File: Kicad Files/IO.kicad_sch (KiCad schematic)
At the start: 1 part, among them U46 RP2040

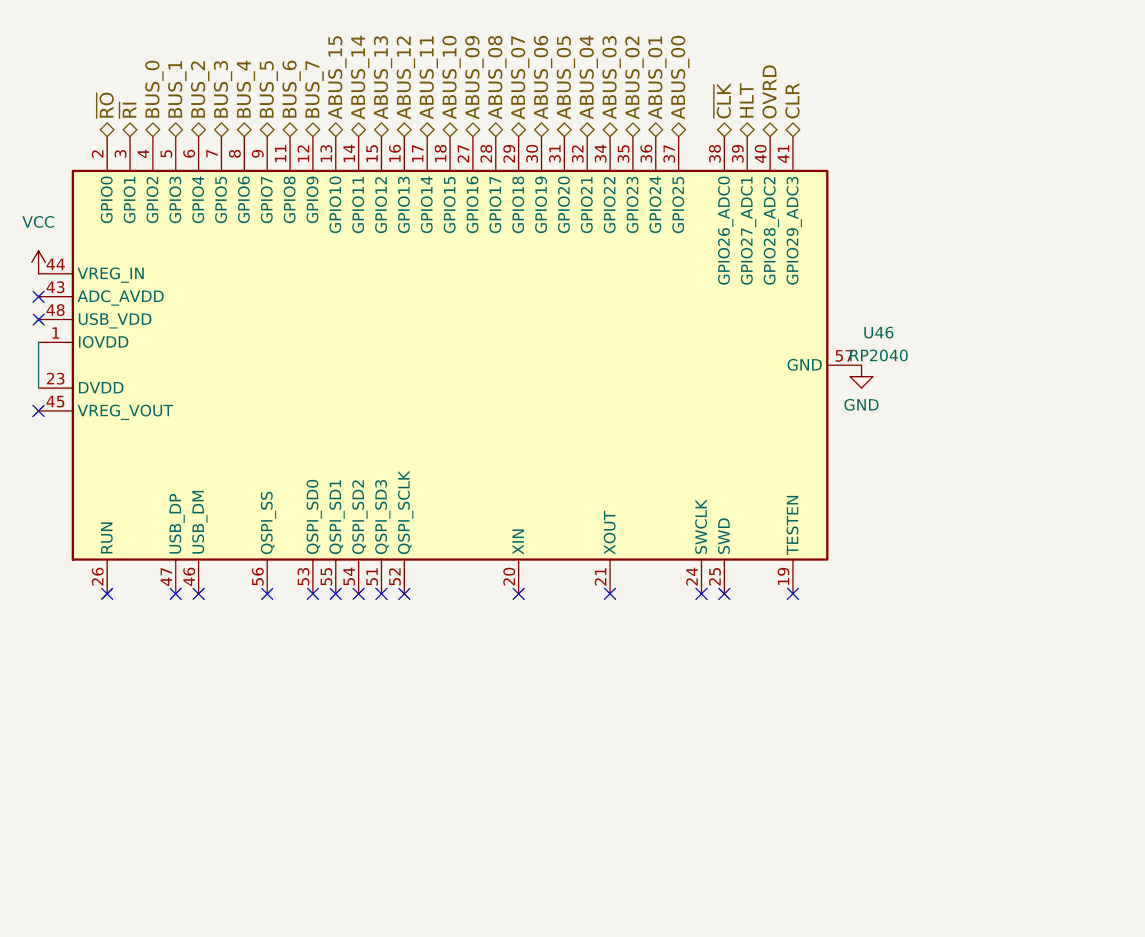
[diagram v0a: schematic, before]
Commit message: im sooo stupiiid
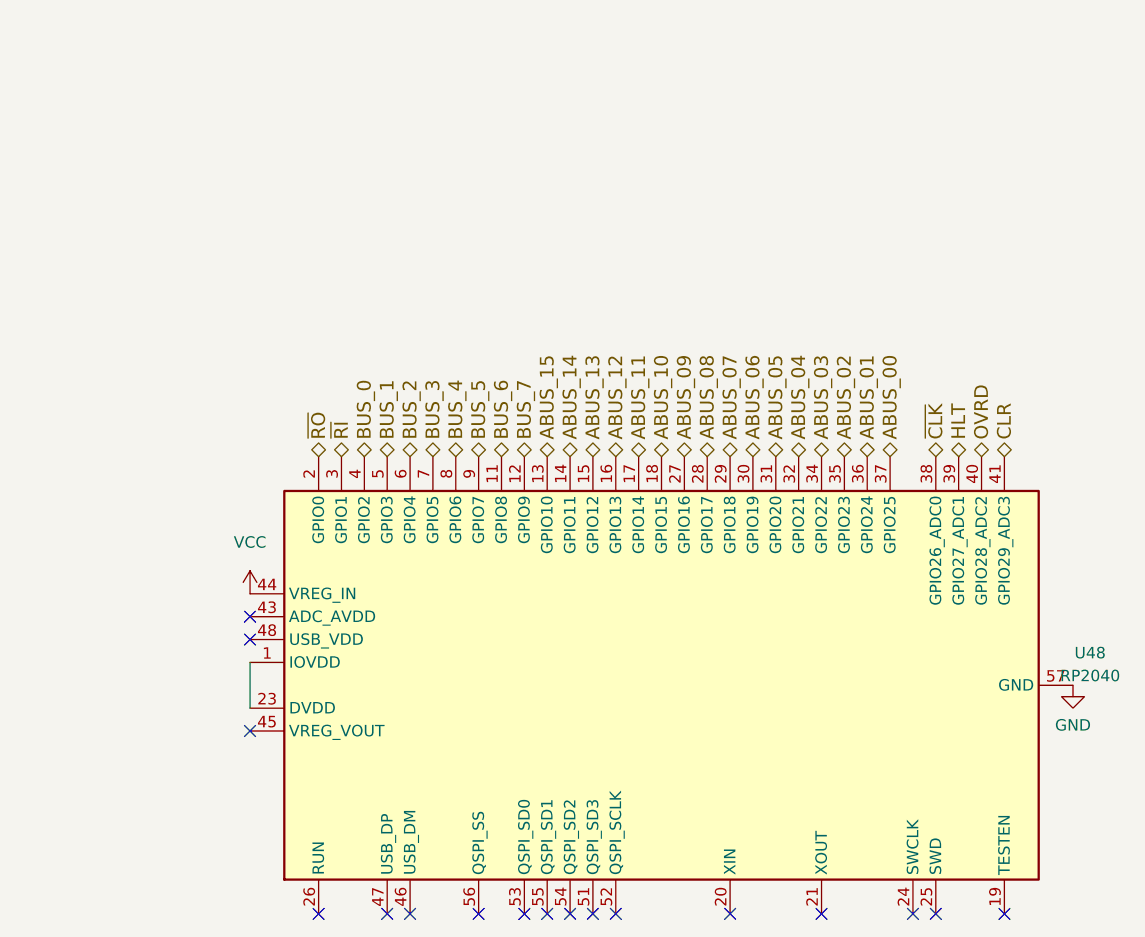
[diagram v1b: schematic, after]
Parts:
- renumbered U46 to U48
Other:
- moved on the sheet: U48
